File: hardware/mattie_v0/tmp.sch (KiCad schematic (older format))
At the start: 52 parts, among them J10 DACS, J11 SERV_0, J12 SERV_1, J13 SERV_2, J14 SERV_3, J15 SERV_4, J16 SERV_5, J17 SERV_6, J18 SERV_7, J19 CAN, J20 USB_B_Mini, J4 GPIO1, J5 GPIO2, J6 GPIO3, P1 SWD, SW2 BOOT0, U4 BMI160, U5 STM32F405RGTx, U6 TJA1051TK-3, Y1 8Mhz

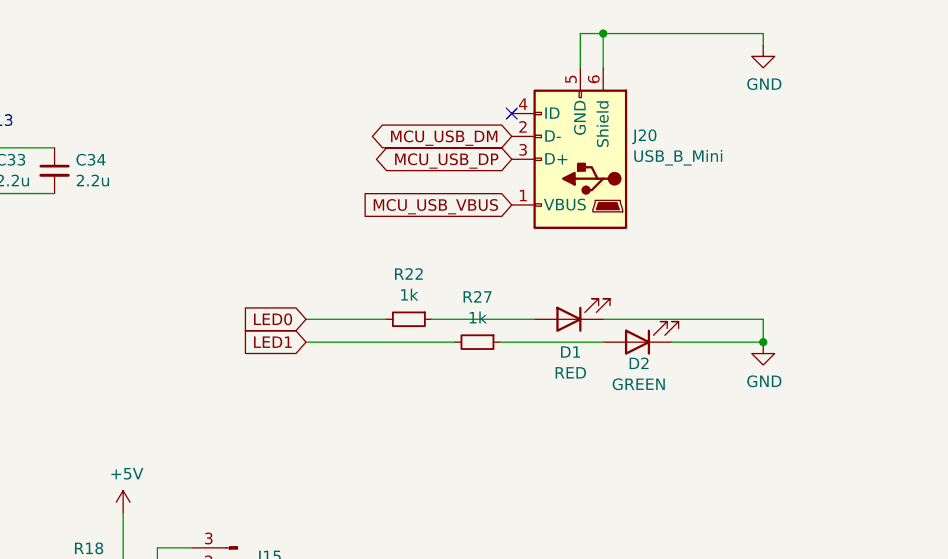
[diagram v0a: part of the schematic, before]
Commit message: update
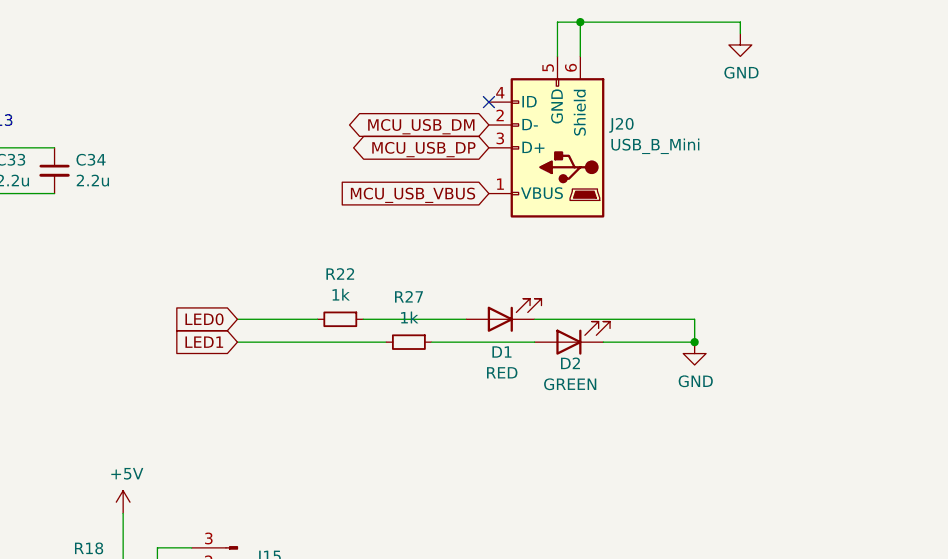
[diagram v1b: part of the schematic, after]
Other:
- moved on the sheet: D1, D2, J20, R22, R27
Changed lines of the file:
@@
 L Device:R_Small R22
 U 1 1 5D85C4C3
-P 8950 2200
-F 0 "R22" V 8754 2200 50  0000 C CNN
-F 1 "1k" V 8845 2200 50  0000 C CNN
-F 2 "Resistor_SMD:R_0603_1608Metric" H 8950 2200 50  0001 C CNN
-F 3 "~" H 8950 2200 50  0001 C CNN
-F 4 " 311-1.00KHRCT-ND " H 8950 2200 50  0001 C CNN "OrderN"
-	1    8950 2200
+P 8650 2200
+F 0 "R22" V 8454 2200 50  0000 C CNN
+F 1 "1k" V 8545 2200 50  0000 C CNN
+F 2 "Resistor_SMD:R_0603_1608Metric" H 8650 2200 50  0001 C CNN
+F 3 "~" H 8650 2200 50  0001 C CNN
+F 4 " 311-1.00KHRCT-ND " H 8650 2200 50  0001 C CNN "OrderN"
+	1    8650 2200
 	0    1    1    0
 $EndComp
@@
 L Device:LED D2
 U 1 1 5D84A7A7
-P 9950 2300
-F 0 "D2" H 9943 2395 50  0000 C CNN
-F 1 "GREEN" H 9943 2486 50  0000 C CNN
-F 2 "LED_SMD:LED_0603_1608Metric" H 9950 2300 50  0001 C CNN
-F 3 "~" H 9950 2300 50  0001 C CNN
-F 4 "160-1446-1-ND " H 9950 2300 50  0001 C CNN "OrderN"
-	1    9950 2300
+P 9650 2300
+F 0 "D2" H 9643 2395 50  0000 C CNN
+F 1 "GREEN" H 9643 2486 50  0000 C CNN
+F 2 "LED_SMD:LED_0603_1608Metric" H 9650 2300 50  0001 C CNN
+F 3 "~" H 9650 2300 50  0001 C CNN
+F 4 "160-1446-1-ND " H 9650 2300 50  0001 C CNN "OrderN"
+	1    9650 2300
 	-1   0    0    1
 $EndComp
@@
 L Device:LED D1
 U 1 1 5D849E88
-P 9650 2200
-F 0 "D1" H 9643 2345 50  0000 C CNN
-F 1 "RED" H 9643 2436 50  0000 C CNN
-F 2 "LED_SMD:LED_0603_1608Metric" H 9650 2200 50  0001 C CNN
-F 3 "~" H 9650 2200 50  0001 C CNN
-F 4 "SML-D12U1WT86CT-ND " H 9650 2200 50  0001 C CNN "OrderN"
-	1    9650 2200
+P 9350 2200
+F 0 "D1" H 9343 2345 50  0000 C CNN
+F 1 "RED" H 9343 2436 50  0000 C CNN
+F 2 "LED_SMD:LED_0603_1608Metric" H 9350 2200 50  0001 C CNN
+F 3 "~" H 9350 2200 50  0001 C CNN
+F 4 "SML-D12U1WT86CT-ND " H 9350 2200 50  0001 C CNN "OrderN"
+	1    9350 2200
 	-1   0    0    1
 $EndComp
@@
 L power:GND #PWR047
 U 1 1 5D849679
-P 10500 2300
-F 0 "#PWR047" H 10500 2050 50  0001 C CNN
-F 1 "GND" H 10505 2127 50  0000 C CNN
-F 2 "" H 10500 2300 50  0001 C CNN
-F 3 "" H 10500 2300 50  0001 C CNN
-	1    10500 2300
+P 10200 2300
+F 0 "#PWR047" H 10200 2050 50  0001 C CNN
+F 1 "GND" H 10205 2127 50  0000 C CNN
+F 2 "" H 10200 2300 50  0001 C CNN
+F 3 "" H 10200 2300 50  0001 C CNN
+	1    10200 2300
 	1    0    0    -1
 $EndComp
@@
 L Device:R_Small R27
 U 1 1 5D85D5B6
-P 9250 2300
-F 0 "R27" V 9054 2300 50  0000 C CNN
-F 1 "1k" V 9145 2300 50  0000 C CNN
-F 2 "Resistor_SMD:R_0603_1608Metric" H 9250 2300 50  0001 C CNN
-F 3 "~" H 9250 2300 50  0001 C CNN
-F 4 " 311-1.00KHRCT-ND " H 9250 2300 50  0001 C CNN "OrderN"
-	1    9250 2300
+P 8950 2300
+F 0 "R27" V 8754 2300 50  0000 C CNN
+F 1 "1k" V 8845 2300 50  0000 C CNN
+F 2 "Resistor_SMD:R_0603_1608Metric" H 8950 2300 50  0001 C CNN
+F 3 "~" H 8950 2300 50  0001 C CNN
+F 4 " 311-1.00KHRCT-ND " H 8950 2300 50  0001 C CNN "OrderN"
+	1    8950 2300
 	0    1    1    0
 $EndComp
@@
 	0    1    1    0
 $EndComp
-NoConn ~ 9400 1300
+NoConn ~ 9300 1250
 $Comp
 L power:GND #PWR046
 U 1 1 5D88B2F0
-P 10500 1000
-F 0 "#PWR046" H 10500 750 50  0001 C CNN
-F 1 "GND" H 10505 827 50  0000 C CNN
-F 2 "" H 10500 1000 50  0001 C CNN
-F 3 "" H 10500 1000 50  0001 C CNN
-	1    10500 1000
-	1    0    0    -1
-$EndComp
-Text GLabel 9400 1700 0    50   Input ~ 0
+P 10400 950
+F 0 "#PWR046" H 10400 700 50  0001 C CNN
+F 1 "GND" H 10405 777 50  0000 C CNN
+F 2 "" H 10400 950 50  0001 C CNN
+F 3 "" H 10400 950 50  0001 C CNN
+	1    10400 950
+	1    0    0    -1
+$EndComp
+Text GLabel 9300 1650 0    50   Input ~ 0
 MCU_USB_VBUS
-Text GLabel 9400 1400 0    50   BiDi ~ 0
+Text GLabel 9300 1350 0    50   BiDi ~ 0
 MCU_USB_DM
-Text GLabel 9400 1500 0    50   BiDi ~ 0
+Text GLabel 9300 1450 0    50   BiDi ~ 0
 MCU_USB_DP
 Wire Wire Line
@@
 L Connector:USB_B_Mini J20
 U 1 1 5D8865AF
-P 9700 1500
-F 0 "J20" H 9470 1397 50  0000 R CNN
-F 1 "USB_B_Mini" H 9470 1488 50  0000 R CNN
-F 2 "Connector_USB:USB_Mini-B_Lumberg_2486_01_Horizontal" H 9850 1450 50  0001 C CNN
-F 3 "~" H 9850 1450 50  0001 C CNN
-F 4 " 151-1206-1-ND " H 9700 1500 50  0001 C CNN "OrderN"
-	1    9700 1500
+P 9600 1450
+F 0 "J20" H 9370 1347 50  0000 R CNN
+F 1 "USB_B_Mini" H 9370 1438 50  0000 R CNN
+F 2 "Connector_USB:USB_Mini-B_Lumberg_2486_01_Horizontal" H 9750 1400 50  0001 C CNN
+F 3 "~" H 9750 1400 50  0001 C CNN
+F 4 " 151-1206-1-ND " H 9600 1450 50  0001 C CNN "OrderN"
+	1    9600 1450
 	-1   0    0    1
 $EndComp
 Wire Wire Line
-	9800 1100 9800 950
-Wire Wire Line
-	9800 950  10500 950
-Wire Wire Line
-	10500 950  10500 1000
-Wire Wire Line
-	9700 1100 9700 950
-Wire Wire Line
-	9700 950  9800 950
-Connection ~ 9800 950
+	9700 1050 9700 900
+Wire Wire Line
+	9700 900  10400 900
+Wire Wire Line
+	10400 900  10400 950
+Wire Wire Line
+	9600 1050 9600 900
+Wire Wire Line
+	9600 900  9700 900
+Connection ~ 9700 900
 $Comp
 L Device:C_Small C34
@@
 	4150 5000 4150 5100
 Wire Wire Line
-	8500 2200 8850 2200
-Wire Wire Line
-	9050 2200 9500 2200
-Wire Wire Line
-	10500 2200 10500 2300
-Wire Wire Line
-	10500 2300 10100 2300
-Connection ~ 10500 2300
-Wire Wire Line
-	9800 2300 9350 2300
-Wire Wire Line
-	9150 2300 8500 2300
+	8200 2200 8550 2200
+Wire Wire Line
+	8750 2200 9200 2200
+Wire Wire Line
+	10200 2200 10200 2300
+Wire Wire Line
+	10200 2300 9800 2300
+Connection ~ 10200 2300
+Wire Wire Line
+	9500 2300 9050 2300
+Wire Wire Line
+	8850 2300 8200 2300
 NoConn ~ 4950 3100
 Wire Wire Line
@@
 Text GLabel 3550 4300 0    50   Input ~ 0
 LED0
-Text GLabel 8500 2200 0    50   Input ~ 0
+Text GLabel 8200 2200 0    50   Input ~ 0
 LED0
 Text GLabel 3550 4400 0    50   Input ~ 0
 LED1
-Text GLabel 8500 2300 0    50   Input ~ 0
+Text GLabel 8200 2300 0    50   Input ~ 0
 LED1
 Wire Wire Line
 	4950 2800 5800 2800
 Wire Wire Line
-	9800 2200 10500 2200
+	9500 2200 10200 2200
 $Comp
 L power:GND #PWR036
